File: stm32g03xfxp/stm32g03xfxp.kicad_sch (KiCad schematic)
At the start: 17 parts, among them J1 USB2.0_C_v3, J3 ProMicro-RightPin, SW1 SW_Push, U2 AMS1117-3.3, U2 STM32G030F6Px

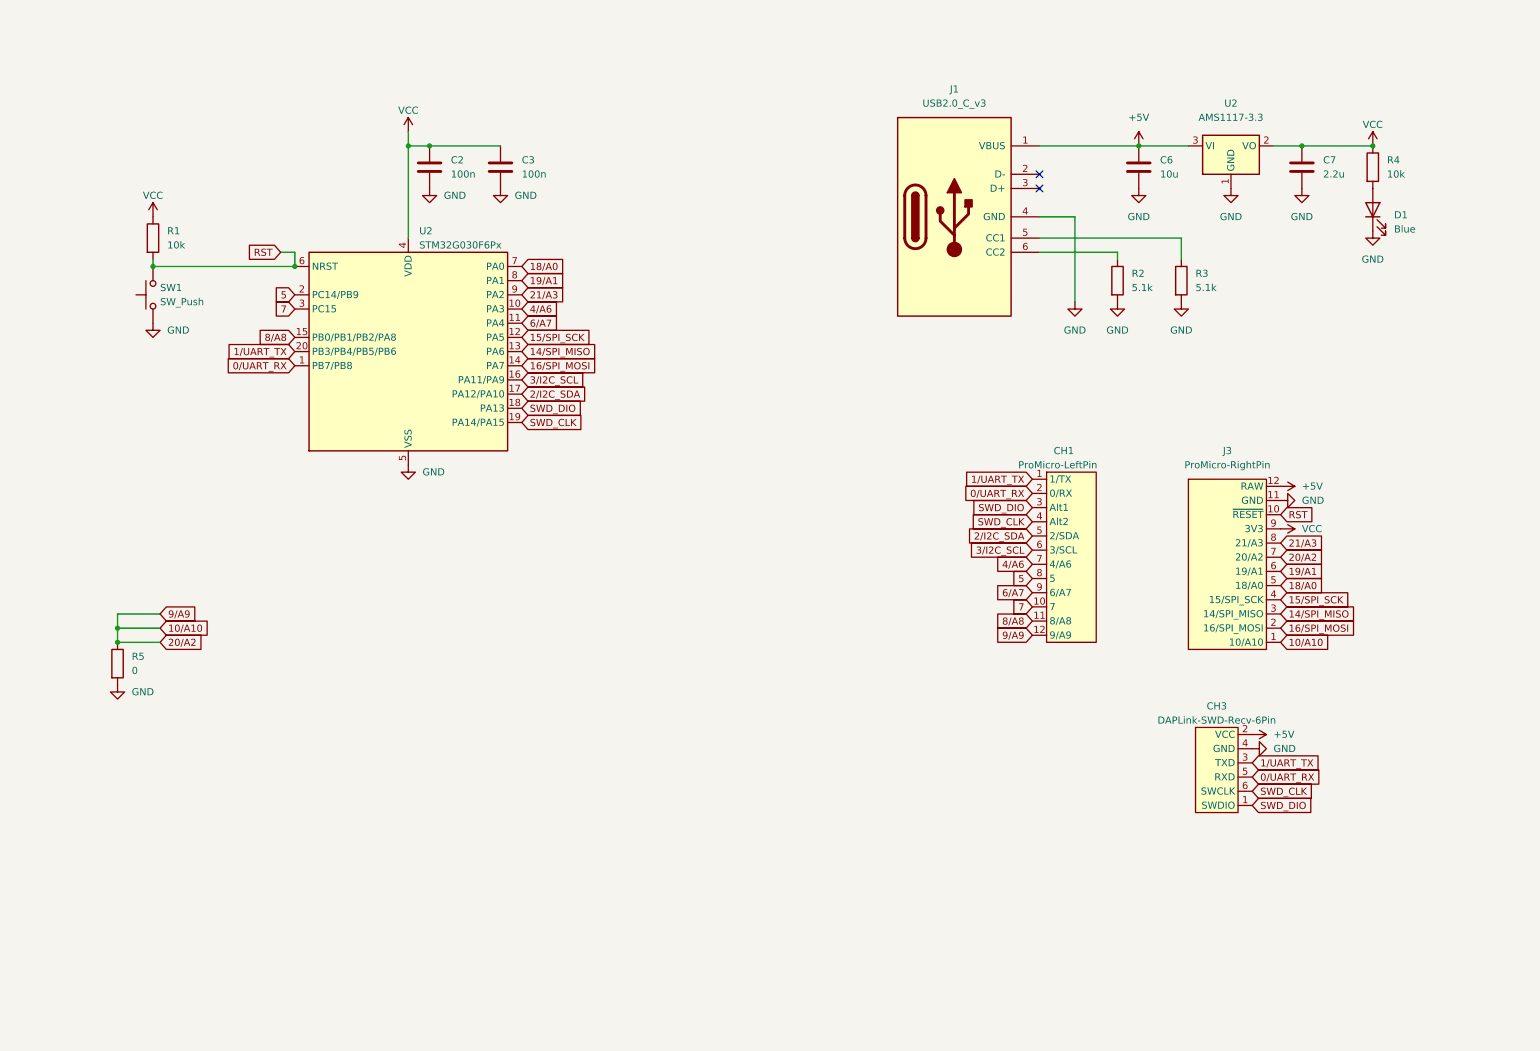
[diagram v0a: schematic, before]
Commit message: stm32g03xfxp/v1.2.0
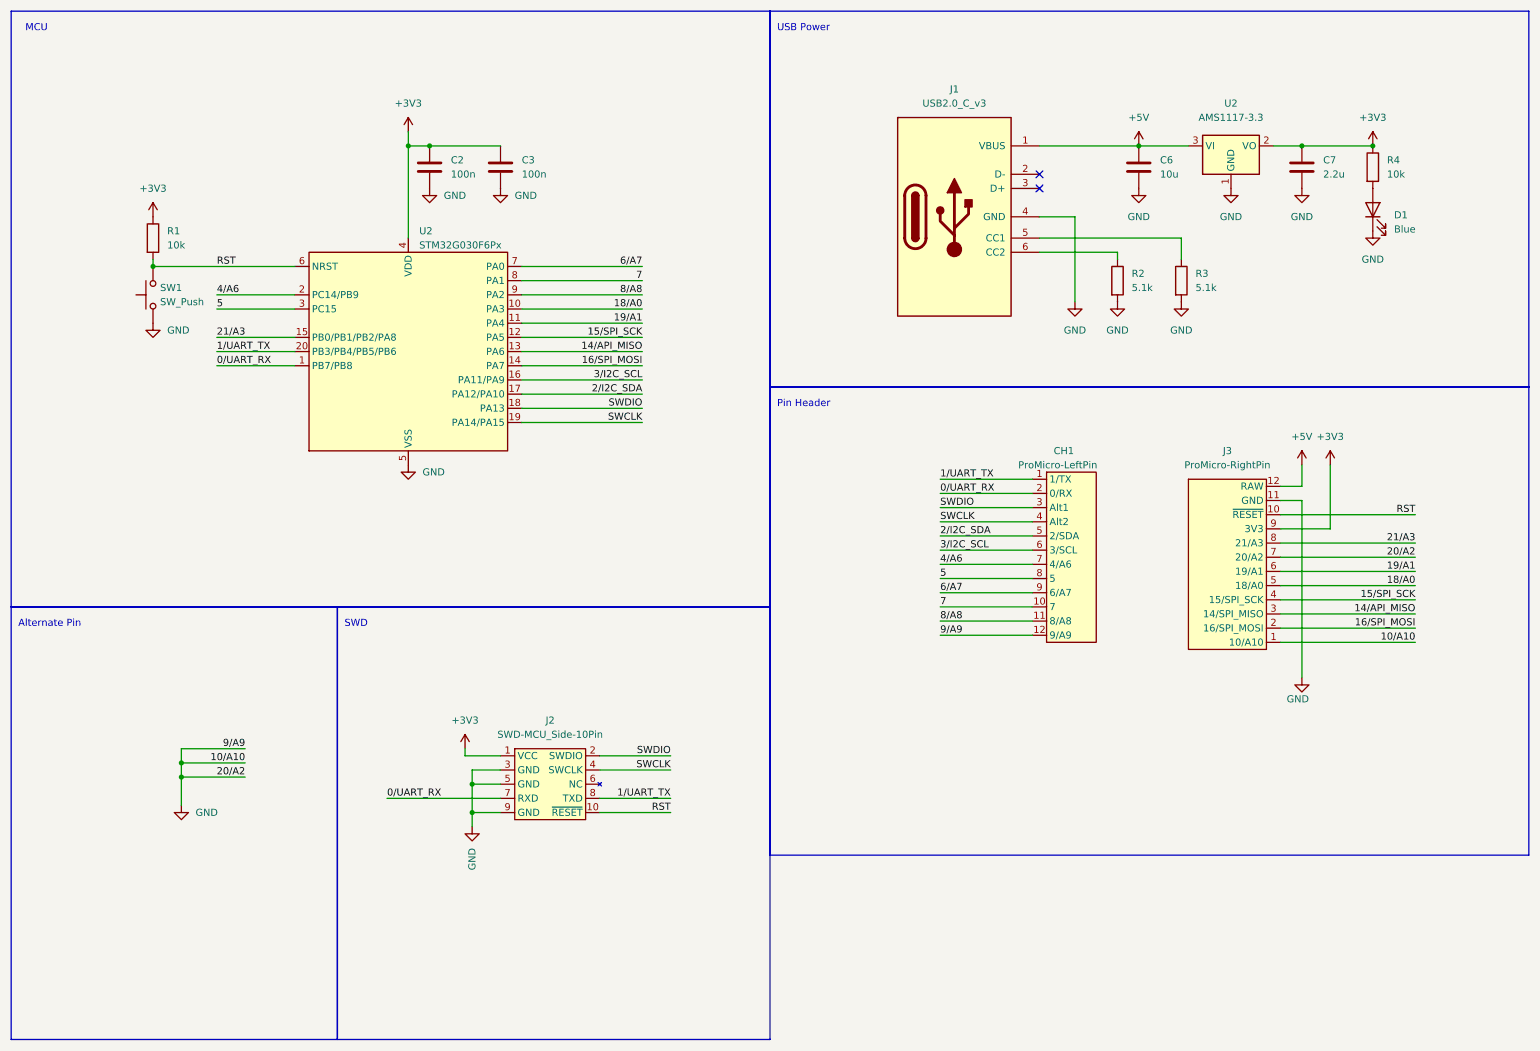
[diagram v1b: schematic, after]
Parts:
- removed CH3: DAPLink-SWD-Recv-6Pin, $74th:BoxPinHeader_2x03_P1.27mm_Vertical, symbol $74th:DAPLink-SWD-Recv-6Pin
- removed R5: 0, $74th:Register_0805_2012, symbol Device:R
- added J2: SWD-MCU_Side-10Pin, $74th:SWD_2x05_P1.27mm, symbol $74th:SWD-MCU_Side-10Pin
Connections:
- net 10/A10 is gone; now on net GND: CH1.12 (9/A9), J3.1 (10/A10), J3.7 (20/A2)
- net 0/UART_RX: now also J2.7 (RXD)
- net 18/A0: now also U2.10 (PA3); no longer U2.7 (PA0)
- net 19/A1: now also U2.11 (PA4); no longer U2.8 (PA1)
- net 1/UART_TX: now also J2.8 (TXD)
- net 21/A3: now also U2.15 (PB0/PB1/PB2/PA8); no longer U2.9 (PA2)
- net 4/A6: now also U2.2 (PC14/PB9); no longer U2.10 (PA3)
- net 5: now also U2.3 (PC15); no longer U2.2 (PC14/PB9)
- net 6/A7: now also U2.7 (PA0); no longer U2.11 (PA4)
- net 7: now also U2.8 (PA1); no longer U2.3 (PC15)
- net 8/A8: now also U2.9 (PA2); no longer U2.15 (PB0/PB1/PB2/PA8)
- net GND: now also J2.3 (GND), J2.5 (GND), J2.9 (GND)
- net RST: now also J2.10 (~{RESET})
- net 14/SPI_MISO renamed 14/API_MISO
- net SWD_CLK renamed SWCLK
- net SWCLK: now also J2.4 (SWCLK)
- net SWD_DIO renamed SWDIO
- net SWDIO: now also J2.2 (SWDIO)
- net VCC renamed +3V3
- net +3V3: now also J2.1 (VCC)
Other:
- note added: "Alternate Pin"
- note added: "MCU"
- note added: "Pin Header"
- note added: "SWD"
- note added: "USB Power"
